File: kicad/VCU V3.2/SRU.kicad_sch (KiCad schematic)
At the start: 5 parts, among them U9 LTV-817S

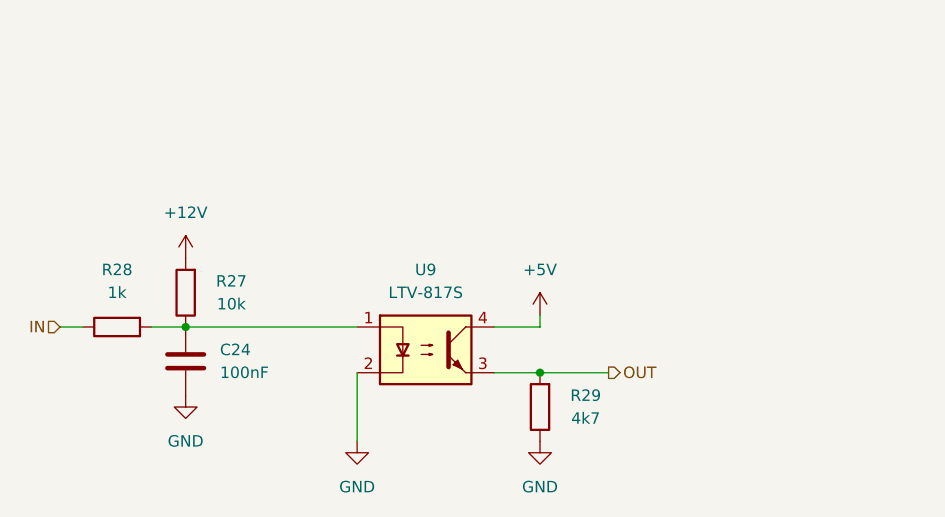
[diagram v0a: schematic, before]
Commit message: VCU V3.2
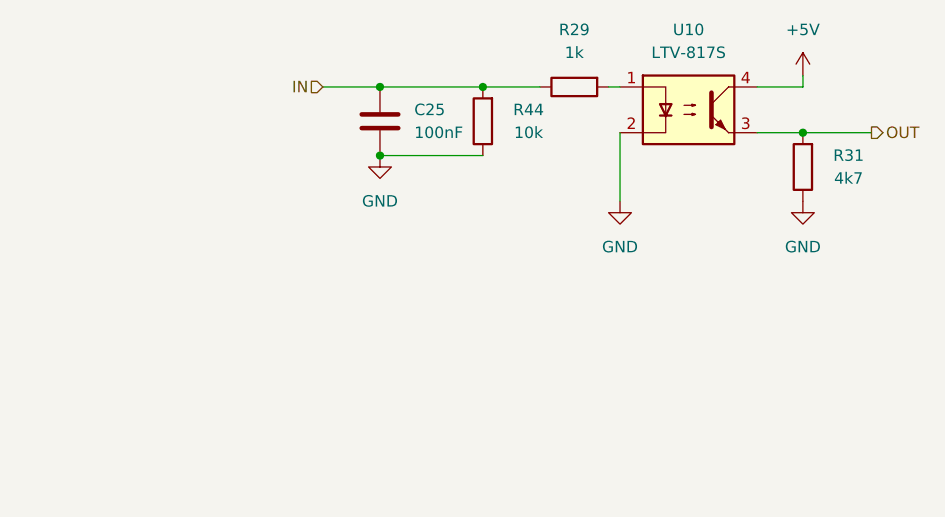
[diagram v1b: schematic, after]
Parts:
- removed R27: 10k, symbol Device:R
- added R44: 10k, symbol Device:R
- renumbered C24 to C25, R28 to R29, R29 to R31, U9 to U10
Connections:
- net GND: now also R44.1
- net IN: now also C25.1, R44.2
- net at R29.2, U10.1: no longer C25.1
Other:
- moved on the sheet: C25, R29, R31, U10

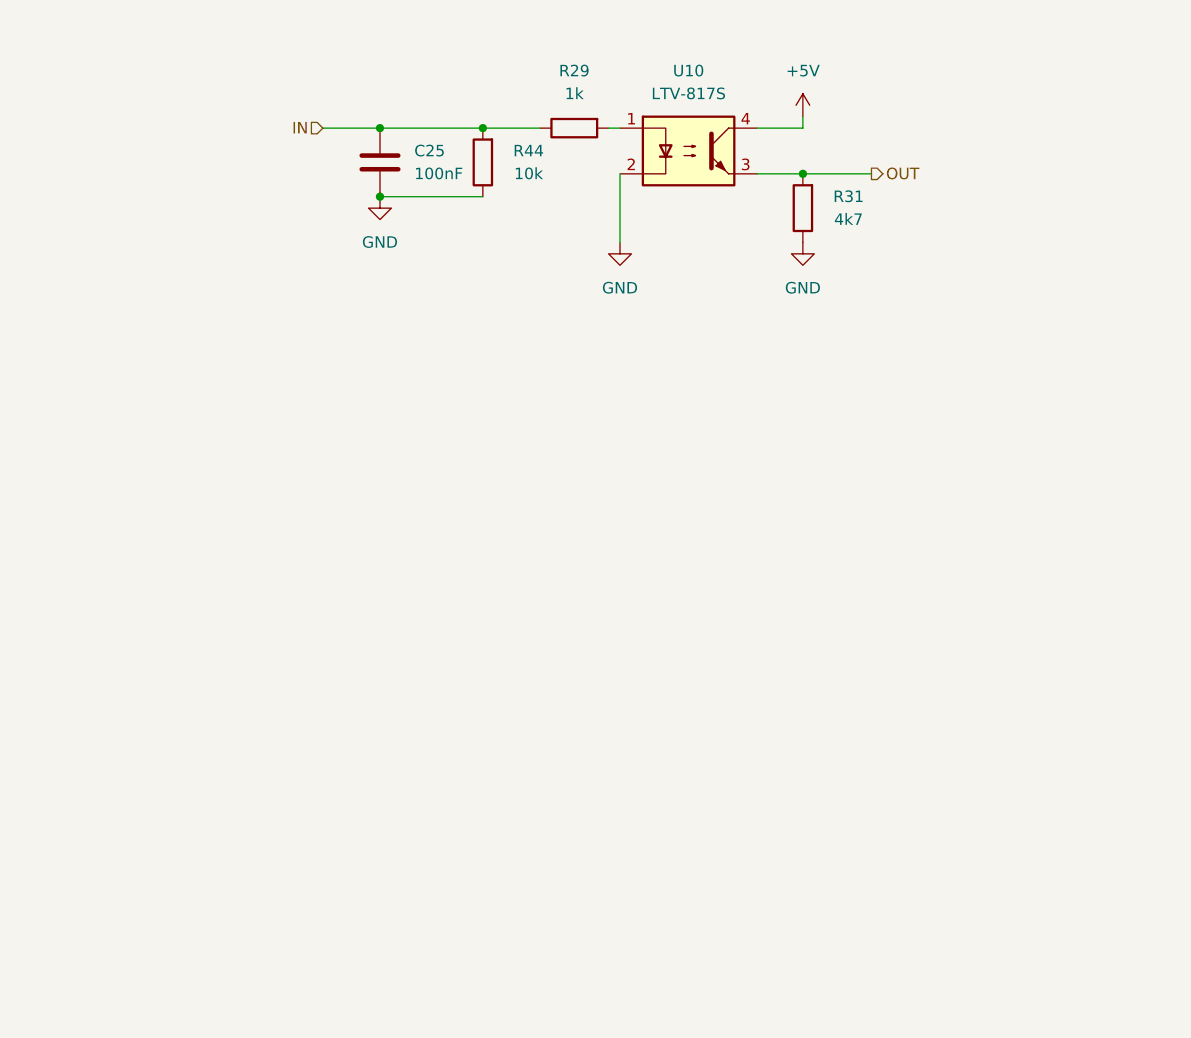
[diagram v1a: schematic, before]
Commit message: vcuv3.2 haha where
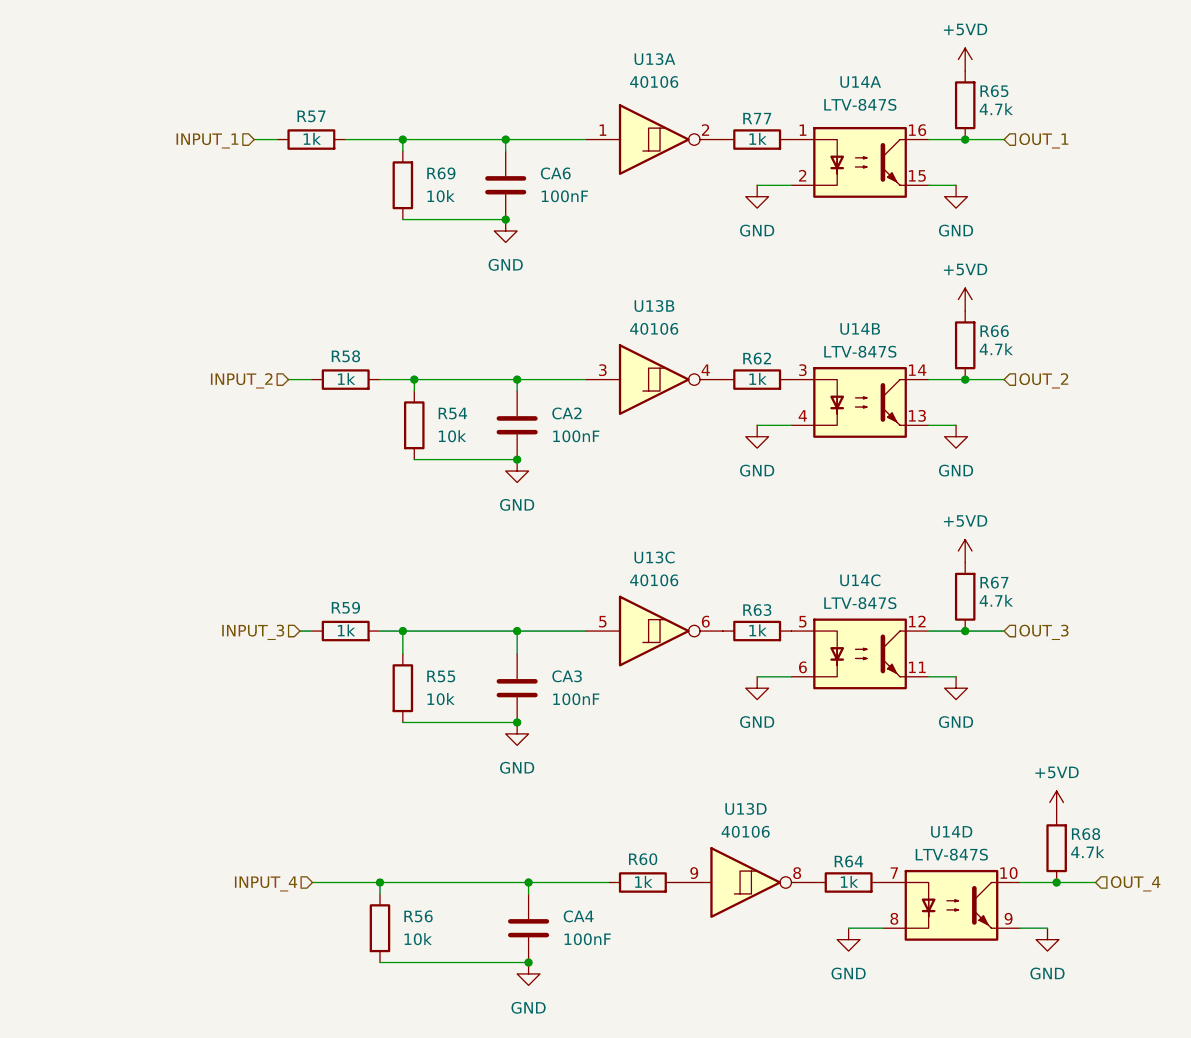
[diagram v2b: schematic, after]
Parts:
- removed C25: 100nF, symbol Device:C
- removed R29: 1k, symbol Device:R
- removed R31: 4k7, symbol Device:R
- removed R44: 10k, symbol Device:R
- removed U10: LTV-817S, Package_DIP:SMDIP-4_W9.53mm, symbol Isolator:LTV-817S
- added CA2, CA3, CA4, CA6: 100nF, RMC_Capacitor:C_0805_2012Metric_Pad1.18x1.45mm_HandSolder_L, symbol Device:C
- added R54, R55, R56, R69: 10k, RMC_Resistor:R_0805_2012Metric_Pad1.20x1.40mm_HandSolder_L, symbol Device:R
- added R57, R58, R59, R60, R62, R63, R64, R77: 1k, RMC_Resistor:R_0805_2012Metric_Pad1.20x1.40mm_HandSolder_L, symbol Device:R
- added R65, R66, R67, R68: 4.7k, RMC_Resistor:R_0805_2012Metric_Pad1.20x1.40mm_HandSolder_L, symbol Device:R
- added U13: 40106, CD40106BMT:SOIC127P600X175-14N, symbol 4xxx:40106
- added U14: LTV-847S, Package_DIP:SMDIP-16_W9.53mm, symbol Isolator:LTV-847S
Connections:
- net GND: now also CA2.2, CA3.2, CA4.2, CA6.1, R54.2, R55.2, R56.2, R69.1, U14.11, U14.13, U14.15, U14.2, U14.4, U14.6, U14.8, U14.9
- new net: CA6.2, R57.2, R69.2, U13.1
- new net: CA3.1, R55.1, R59.2, U13.5
- new net: CA2.1, R54.1, R58.2, U13.3
- new net: R63.1, U13.6
- new net: R63.2, U14.5
- new net: R64.1, U13.8
- new net: R64.2, U14.7
- new net: R62.1, U13.4
- new net: R60.2, U13.9
- new net: R62.2, U14.3
- new net: R77.2, U14.1
- new net: R77.1, U13.2
- new net +5VD: R65.2, R66.2, R67.2, R68.2
- new net INPUT_1: R57.1
- new net INPUT_2: R58.1
- new net INPUT_3: R59.1
- new net INPUT_4: CA4.1, R56.1, R60.1
- new net OUT_1: R65.1, U14.16
- new net OUT_2: R66.1, U14.14
- new net OUT_3: R67.1, U14.12
- new net OUT_4: R68.1, U14.10
